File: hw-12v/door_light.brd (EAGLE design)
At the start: 26.2 x 28.6 mm, 24 parts, among them IC1 TINY13-20SSU, IC2 78L05F, T1 IRFML8244, T2 IRFML8244, T3 KP-3216P3C

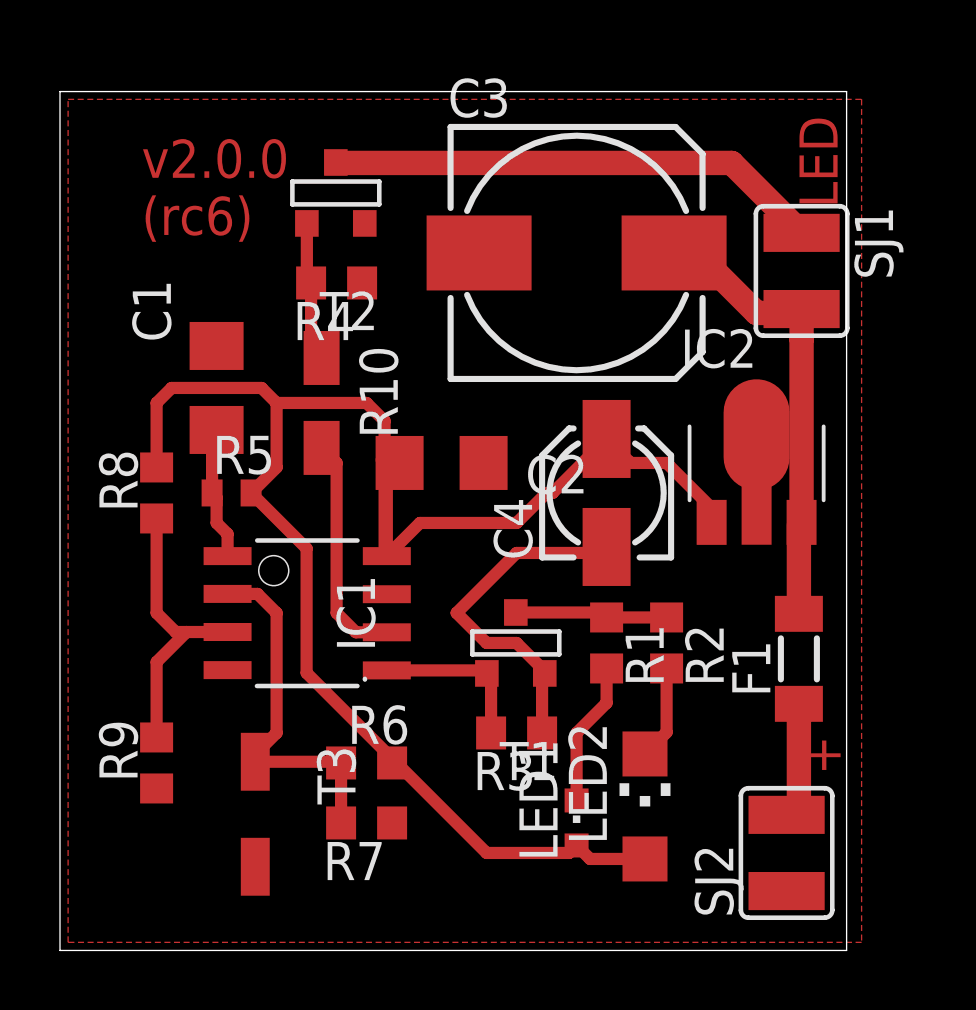
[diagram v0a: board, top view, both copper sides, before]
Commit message: elements are now more compact
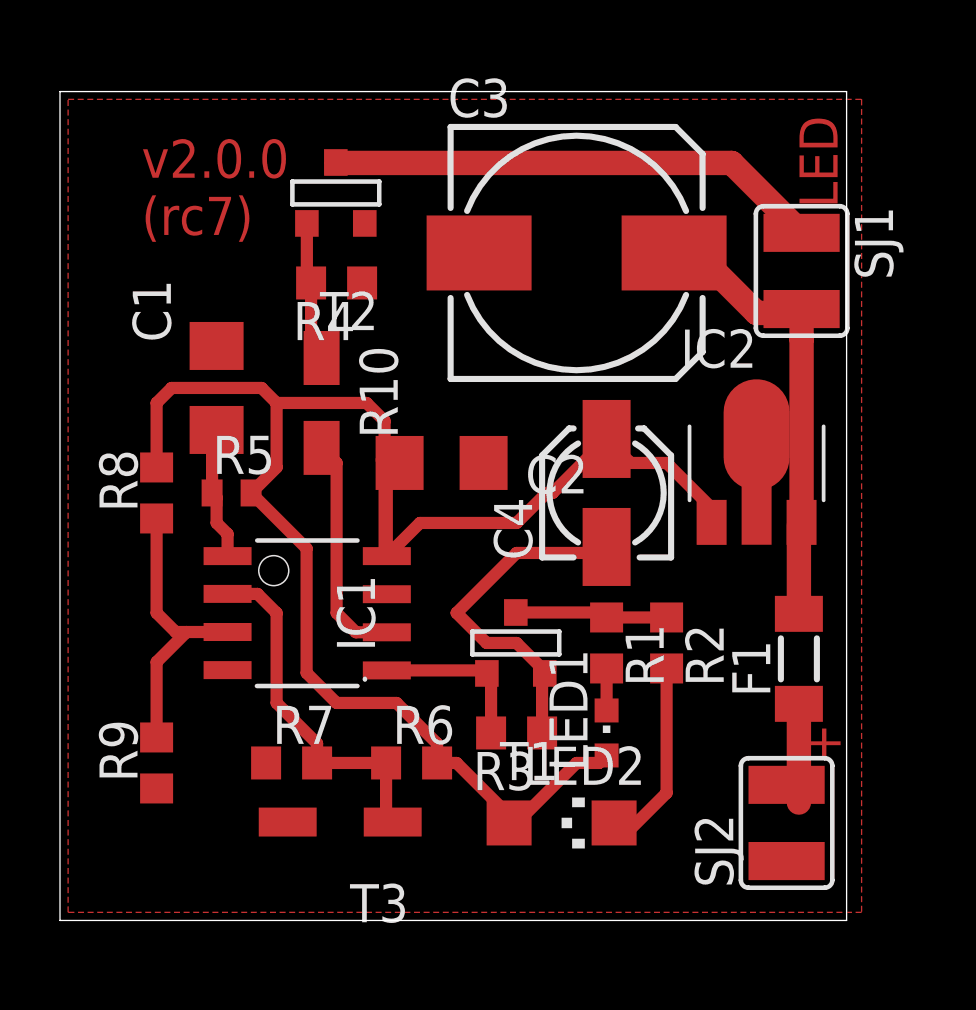
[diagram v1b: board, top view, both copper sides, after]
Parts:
- moved T3 3.68 mm to (32.5, 45.5), turned to 180 degrees
- moved R7 3.20 mm to (30.5, 47.0), turned to 0 degrees
- moved LED1 3.16 mm to (41.0, 48.0)
- moved LED2 2.83 mm to (39.5, 45.0), turned to 270 degrees
- moved R6 1.50 mm to (34.5, 47.0)
- moved SJ2 1.00 mm to (47.0, 45.0)
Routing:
- net N$1: track 4.81 -> 1.40 mm
- net N$2: track 3.15 -> 6.51 mm
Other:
- board size 26.2 x 28.6 mm -> 26.2 x 27.6 mm
- board text added: "v2.0.0 (rc7)"
- board text removed: "v2.0.0 (rc6)"
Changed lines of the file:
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@@
 <board>
 <plain>
-<wire x1="22.78" y1="40.75" x2="49" y2="40.75" width="0" layer="20"/>
-<wire x1="49" y1="40.75" x2="49" y2="69.38" width="0" layer="20"/>
+<wire x1="22.78" y1="41.75" x2="49" y2="41.75" width="0" layer="20"/>
+<wire x1="49" y1="41.75" x2="49" y2="69.38" width="0" layer="20"/>
 <wire x1="49" y1="69.38" x2="22.78" y2="69.38" width="0" layer="20"/>
-<wire x1="22.78" y1="69.38" x2="22.78" y2="40.75" width="0" layer="20"/>
-<text x="48.8" y="46.6" size="1.27" layer="1" rot="R90">+</text>
+<wire x1="22.78" y1="69.38" x2="22.78" y2="41.75" width="0" layer="20"/>
+<text x="48.8" y="47" size="1.27" layer="1" rot="R90">+</text>
 <text x="48.7" y="65.5" size="1.27" layer="1" rot="R90">LED</text>
 <text x="25.5" y="64.6" size="1.27" layer="1">v2.0.0
-(rc6)</text>
+(rc7)</text>
 </plain>
 <attributes>
@@
 <element name="F1" library="rcl" package="MINI_MELF-0204W" value="F750mA" x="47.41" y="50.47" rot="R90"/>
 <element name="R5" library="rcl" package="R0402" value="10kR" x="28.5" y="56"/>
-<element name="R7" library="rcl" package="R0603" value="2.7kR" x="33" y="45" rot="R180"/>
+<element name="R7" library="rcl" package="R0603" value="2.7kR" x="30.5" y="47"/>
 <element name="R8" library="rcl" package="R0603" value="10kR" x="26" y="56" rot="R90"/>
-<element name="R6" library="rcl" package="R0603" value="10kR" x="33" y="47"/>
+<element name="R6" library="rcl" package="R0603" value="10kR" x="34.5" y="47"/>
 <element name="R9" library="rcl" package="R0603" value="2.7kR" x="26" y="47" rot="R90"/>
-<element name="LED2" library="led" package="CHIPLED_1206" value="IR" x="42.28" y="45.55"/>
-<element name="LED1" library="led" package="CHIPLED_0603" value="RED" x="40" y="45"/>
+<element name="LED2" library="led" package="CHIPLED_1206" value="IR" x="39.5" y="45" rot="R270"/>
+<element name="LED1" library="led" package="CHIPLED_0603" value="RED" x="41" y="48"/>
 <element name="R2" library="rcl" package="R0603" value="180R" x="43" y="51" rot="R270"/>
 <element name="R1" library="rcl" package="R0603" value="470R" x="41" y="51" rot="R270"/>
-<element name="T3" library="opto-trans-smd" package="OPTO-TRANS-SIEMENS_BP103" value="KP-3216P3C" x="28.82" y="45.67" rot="R270">
-<attribute name="OC_NEWARK" value="unknown" x="28.82" y="45.67" size="1.778" layer="27" rot="R270" display="off"/>
-<attribute name="MPN" value="" x="28.82" y="45.67" size="1.778" layer="27" rot="R270" display="off"/>
-<attribute name="MF" value="" x="28.82" y="45.67" size="1.778" layer="27" rot="R270" display="off"/>
-<attribute name="OC_FARNELL" value="unknown" x="28.82" y="45.67" size="1.778" layer="27" rot="R270" display="off"/>
+<element name="T3" library="opto-trans-smd" package="OPTO-TRANS-SIEMENS_BP103" value="KP-3216P3C" x="32.5" y="45.5" rot="R180">
+<attribute name="OC_NEWARK" value="unknown" x="32.5" y="45.5" size="1.778" layer="27" rot="R180" display="off"/>
+<attribute name="MPN" value="" x="32.5" y="45.5" size="1.778" layer="27" rot="R180" display="off"/>
+<attribute name="MF" value="" x="32.5" y="45.5" size="1.778" layer="27" rot="R180" display="off"/>
+<attribute name="OC_FARNELL" value="unknown" x="32.5" y="45.5" size="1.778" layer="27" rot="R180" display="off"/>
 </element>
 <element name="T1" library="zetex" package="SOT-23" value="IRFML8244" x="38" y="51" rot="R180">
@@
 <attribute name="OC_FARNELL" value="unknown" x="38" y="51" size="1.778" layer="27" rot="R180" display="off"/>
 </element>
-<element name="SJ2" library="jumper" package="SJW" value="PWR" x="47" y="44" rot="R90"/>
+<element name="SJ2" library="jumper" package="SJW" value="PWR" x="47" y="45" rot="R90"/>
 <element name="SJ1" library="jumper" package="SJW" value="LIGHT" x="47.5" y="63.4" rot="R270"/>
 <element name="R4" library="rcl" package="R0603" value="100kR" x="32" y="63" rot="R180"/>
@@
 <contactref element="C1" pad="2"/>
 <polygon width="0.6096" layer="1" isolate="0.6096" orphans="yes">
-<vertex x="23.05" y="41.02"/>
+<vertex x="23.05" y="42.02"/>
 <vertex x="23.05" y="69.12"/>
 <vertex x="49.5" y="69.12"/>
-<vertex x="49.5" y="41.02"/>
+<vertex x="49.5" y="42.02"/>
 </polygon>
 <contactref element="R7" pad="1"/>
@@
 <contactref element="LED2" pad="C"/>
 <contactref element="R2" pad="2"/>
-<wire x1="43" y1="50.15" x2="43" y2="48.02" width="0.4064" layer="1"/>
-<wire x1="43" y1="48.02" x2="42.28" y2="47.3" width="0.4064" layer="1"/>
+<wire x1="41.25" y1="45" x2="41.72" y2="44.72" width="0.4064" layer="1"/>
+<wire x1="41.72" y1="44.72" x2="43" y2="46" width="0.4064" layer="1"/>
+<wire x1="43" y1="46" x2="43" y2="50.15" width="0.4064" layer="1"/>
 </signal>
 <signal name="N$4">
@@
 <contactref element="SJ2" pad="2"/>
 <wire x1="47.41" y1="48.97" x2="47.41" y2="45.68" width="0.8128" layer="1"/>
-<wire x1="47.41" y1="45.68" x2="47" y2="45.27" width="0.4064" layer="1"/>
+<wire x1="47.41" y1="45.68" x2="47" y2="46.27" width="0.4064" layer="1"/>
 </signal>
 <signal name="N$12">
@@
 <contactref element="IC1" pad="2"/>
 <contactref element="T3" pad="COLLECTOR"/>
-<wire x1="29.29" y1="47.04" x2="29.29" y2="47.29" width="0.4064" layer="1"/>
-<wire x1="29.29" y1="47.29" x2="30" y2="48" width="0.4064" layer="1"/>
-<wire x1="30" y1="48" x2="30" y2="52" width="0.4064" layer="1"/>
-<wire x1="32.15" y1="47" x2="32.15" y2="45" width="0.4064" layer="1"/>
 <wire x1="28.366" y1="52.635" x2="29.365" y2="52.635" width="0.4064" layer="1"/>
 <wire x1="29.365" y1="52.635" x2="30" y2="52" width="0.4064" layer="1"/>
-<wire x1="29.29" y1="47.04" x2="32.11" y2="47.04" width="0.4064" layer="1"/>
-<wire x1="32.11" y1="47.04" x2="32.15" y2="47" width="0.4064" layer="1"/>
+<wire x1="33.61" y1="47.04" x2="33.65" y2="47" width="0.4064" layer="1"/>
+<wire x1="30" y1="52" x2="30" y2="49" width="0.4064" layer="1"/>
+<wire x1="30" y1="49" x2="31.35" y2="47.65" width="0.4064" layer="1"/>
+<wire x1="31.35" y1="47" x2="31.35" y2="47.65" width="0.4064" layer="1"/>
+<wire x1="31.35" y1="47" x2="33.65" y2="47" width="0.4064" layer="1"/>
+<wire x1="33.65" y1="47" x2="33.65" y2="45.1" width="0.4064" layer="1"/>
+<wire x1="33.65" y1="45.1" x2="33.87" y2="45.03" width="0.4064" layer="1"/>
 </signal>
 <signal name="N$17">
@@
 <contactref element="LED1" pad="C"/>
 <contactref element="R1" pad="2"/>
-<wire x1="41" y1="50.15" x2="41" y2="49" width="0.4064" layer="1"/>
-<wire x1="41" y1="49" x2="40" y2="48" width="0.4064" layer="1"/>
-<wire x1="40" y1="48" x2="40" y2="45.75" width="0.4064" layer="1"/>
+<wire x1="41" y1="50.15" x2="41" y2="48.75" width="0.4064" layer="1"/>
 </signal>
 <signal name="N$14">
@@
 <wire x1="43" y1="57" x2="41.8" y2="57" width="0.4064" layer="1"/>
 <wire x1="41.8" y1="57" x2="41" y2="57.8" width="0.4064" layer="1"/>
-<wire x1="42.28" y1="43.8" x2="40.45" y2="43.8" width="0.4064" layer="1"/>
-<wire x1="40.45" y1="43.8" x2="40" y2="44.25" width="0.4064" layer="1"/>
-<wire x1="34" y1="47" x2="33.85" y2="47" width="0.4064" layer="1"/>
-<wire x1="37" y1="44" x2="39.75" y2="44" width="0.4064" layer="1"/>
-<wire x1="39.75" y1="44" x2="40" y2="44.25" width="0.4064" layer="1"/>
-<wire x1="34" y1="47" x2="37" y2="44" width="0.4064" layer="1"/>
-<wire x1="34" y1="47" x2="31" y2="50" width="0.4064" layer="1"/>
 <wire x1="31" y1="50" x2="31" y2="54.15" width="0.4064" layer="1"/>
 <wire x1="26.5" y1="59.5" x2="29.5" y2="59.5" width="0.4064" layer="1"/>
@@
 <wire x1="33.6" y1="58.4" x2="33" y2="59" width="0.4064" layer="1"/>
 <wire x1="33" y1="59" x2="30" y2="59" width="0.4064" layer="1"/>
+<wire x1="31" y1="50" x2="32" y2="49" width="0.4064" layer="1"/>
+<wire x1="32" y1="49" x2="34" y2="49" width="0.4064" layer="1"/>
+<wire x1="34" y1="49" x2="35.35" y2="47.65" width="0.4064" layer="1"/>
+<wire x1="35.35" y1="47" x2="35.35" y2="47.65" width="0.4064" layer="1"/>
+<wire x1="35.35" y1="47" x2="36" y2="47" width="0.4064" layer="1"/>
+<wire x1="36" y1="47" x2="38" y2="45" width="0.4064" layer="1"/>
+<wire x1="38" y1="45" x2="38" y2="44.92" width="0.4064" layer="1"/>
+<wire x1="38" y1="44.92" x2="37.75" y2="45" width="0.4064" layer="1"/>
+<wire x1="38" y1="45" x2="40" y2="47" width="0.4064" layer="1"/>
+<wire x1="40" y1="47" x2="40.75" y2="47" width="0.4064" layer="1"/>
+<wire x1="40.75" y1="47" x2="41" y2="47.25" width="0.4064" layer="1"/>
 </signal>
 <signal name="+12V">
